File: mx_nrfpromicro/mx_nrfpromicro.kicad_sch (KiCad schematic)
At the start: 22 parts, among them SW1 SW_Push_45deg, SW10 SW_Push_45deg, SW11 SW_Push_45deg, SW12 SW_Push_45deg, SW13 SW_Push_45deg, SW14 SW_Push_45deg, SW15 SW_Push_45deg, SW16 SW_Push_45deg, SW17 SW_Push_45deg, SW18 SW_SPDT, SW19 SW_PUSH, SW2 SW_Push_45deg, SW3 SW_Push_45deg, SW4 SW_Push_45deg, SW5 SW_Push_45deg, SW6 SW_Push_45deg, SW7 SW_Push_45deg, SW8 SW_Push_45deg, SW9 SW_Push_45deg, U1 Nice_Nano_V2

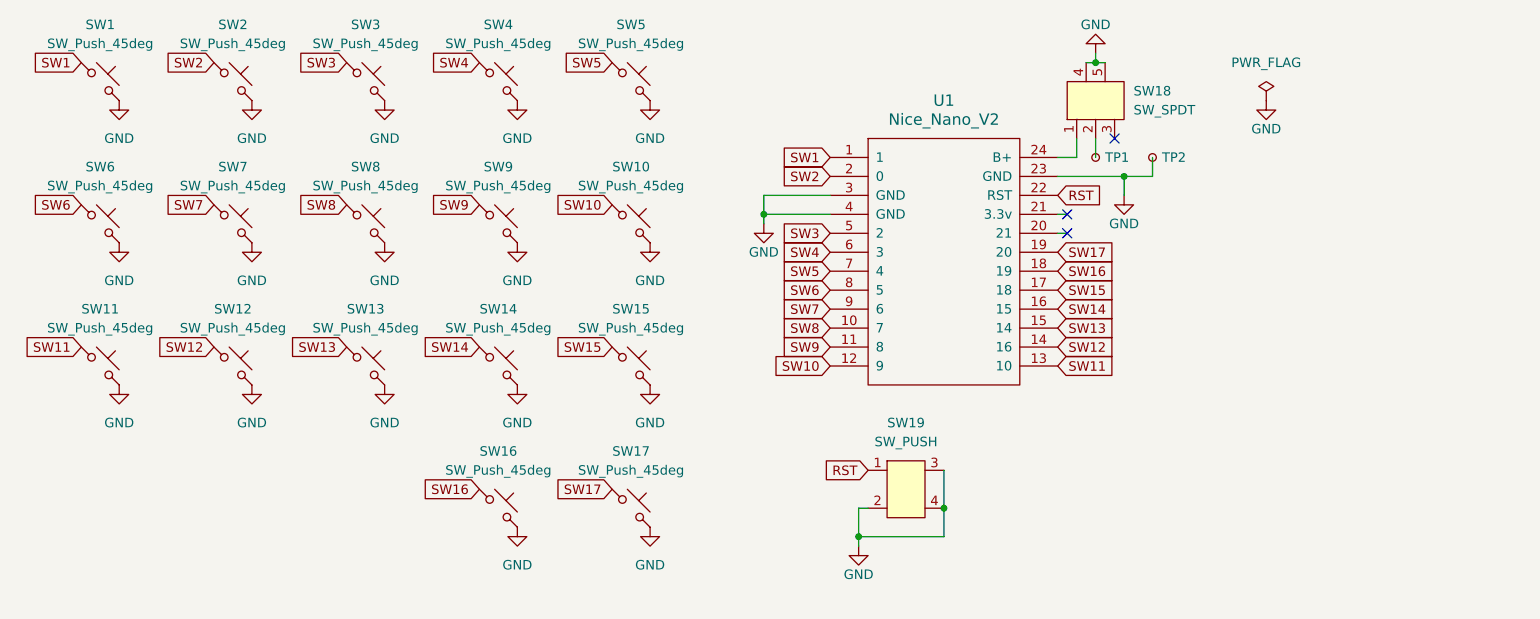
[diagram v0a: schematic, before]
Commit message: updated
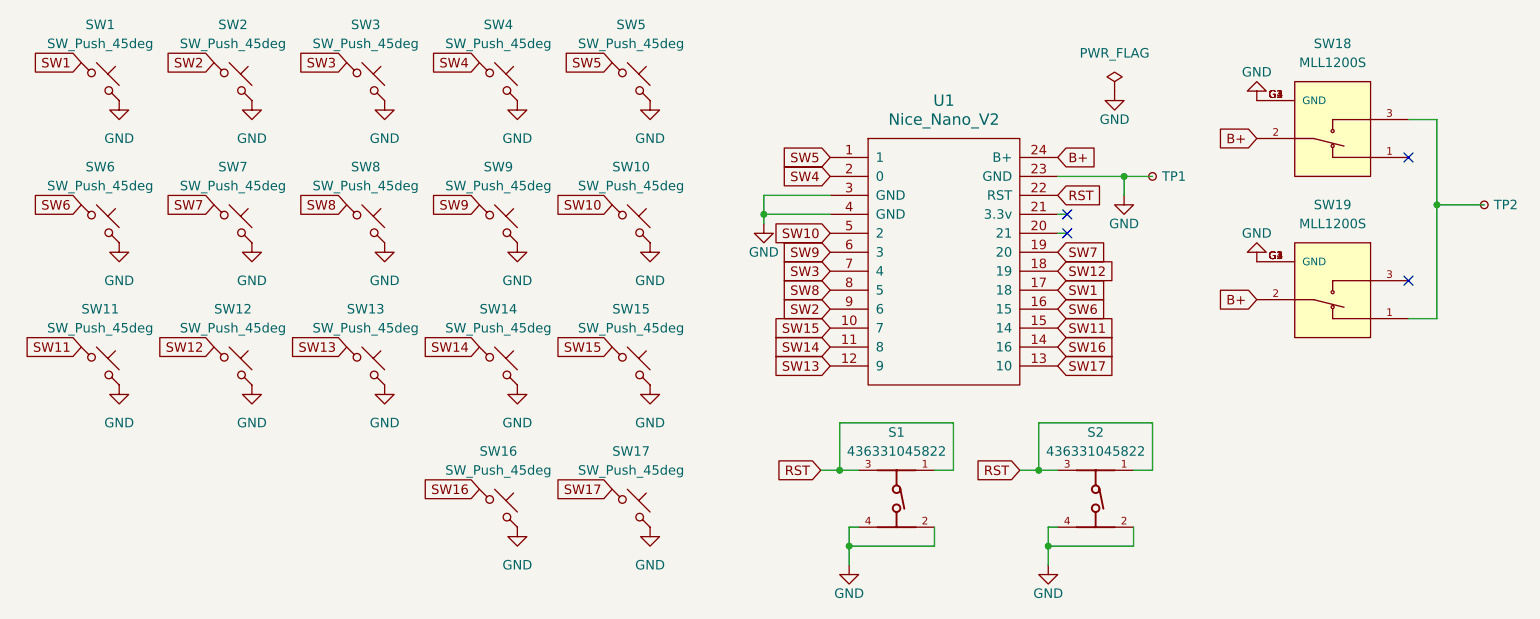
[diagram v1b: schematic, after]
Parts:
- removed SW18: SW_SPDT, BLE_KBD:SS12F23G5, symbol SS12F23G5:SS12F23G5
- removed SW19: SW_PUSH, BLE_KBD:SW_SIDE_MOUNT, symbol SW_SIDE_MOUNT:SW_SIDE_MOUNT
- added S1, S2: 436331045822, BLE_KBD:4363X10458XX, symbol 436331045822:436331045822
- added SW18, SW19: MLL1200S, BLE_KBD:SW_MLL1200S, symbol MLL1200S:MLL1200S
- SW1, SW10, SW11, SW12, SW13, SW14, SW15, SW2, SW3, SW4, SW5, SW6, SW7, SW8, SW9: footprint BLE_KBD:MX_Optional_Reversible_1u -> BLE_KBD:MX_Reversible_Optional_1u
- SW16, SW17: footprint BLE_KBD:MX_Optional_Reversible_1.5u -> BLE_KBD:MX_Reversible_Optional_1.5u
- TP1: renamed from TP2; footprint TestPoint:TestPoint_THTPad_D1.0mm_Drill0.5mm -> TestPoint:TestPoint_THTPad_D1.5mm_Drill0.7mm
- TP2: renamed from TP1; footprint TestPoint:TestPoint_THTPad_D1.0mm_Drill0.5mm -> TestPoint:TestPoint_THTPad_D1.5mm_Drill0.7mm
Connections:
- net GND: now also S1.2, S1.4, S2.2, S2.4, SW18.G1 (GND), SW18.G2 (GND), SW18.G3 (GND), SW18.G4 (GND), SW19.G1 (GND), SW19.G2 (GND), SW19.G3 (GND), SW19.G4 (GND)
- net RST: now also S1.1, S1.3, S2.1, S2.3
- net SW1: now also U1.17 (18); no longer U1.1
- net SW10: now also U1.5 (2); no longer U1.12 (9)
- net SW11: now also U1.15 (14); no longer U1.13 (10)
- net SW12: now also U1.18 (19); no longer U1.14 (16)
- net SW13: now also U1.12 (9); no longer U1.15 (14)
- net SW14: now also U1.11 (8); no longer U1.16 (15)
- net SW15: now also U1.10 (7); no longer U1.17 (18)
- net SW16: now also U1.14 (16); no longer U1.18 (19)
- net SW17: now also U1.13 (10); no longer U1.19 (20)
- net SW2: now also U1.9 (6); no longer U1.2 (0)
- net SW3: now also U1.7 (4); no longer U1.5 (2)
- net SW4: now also U1.2 (0); no longer U1.6 (3)
- net SW5: now also U1.1; no longer U1.7 (4)
- net SW6: now also U1.16 (15); no longer U1.8 (5)
- net SW7: now also U1.19 (20); no longer U1.9 (6)
- net SW8: now also U1.8 (5); no longer U1.10 (7)
- net SW9: now also U1.6 (3); no longer U1.11 (8)
- net B+: now reaches U1.24 (B+)
- net B+: now also SW18.2, SW19.2
- net at TP2.1: now also SW18.3, SW19.1
- no-connect marks 3 -> 4
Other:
- moved on the sheet: TP1, TP2
